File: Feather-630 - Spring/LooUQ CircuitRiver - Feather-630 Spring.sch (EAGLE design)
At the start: 22 parts, among them J1 FEATHERHOST-S, J2 FEATHERHOST-L, J3 HA-CTA_HEADER, J4 JST_PH-2_T/H, J5 JST_PH-2_T/H, P1 NO MOUNT, P2 NO MOUNT, P3 BREAKOUTPAD, U2 LM2674_BUCK

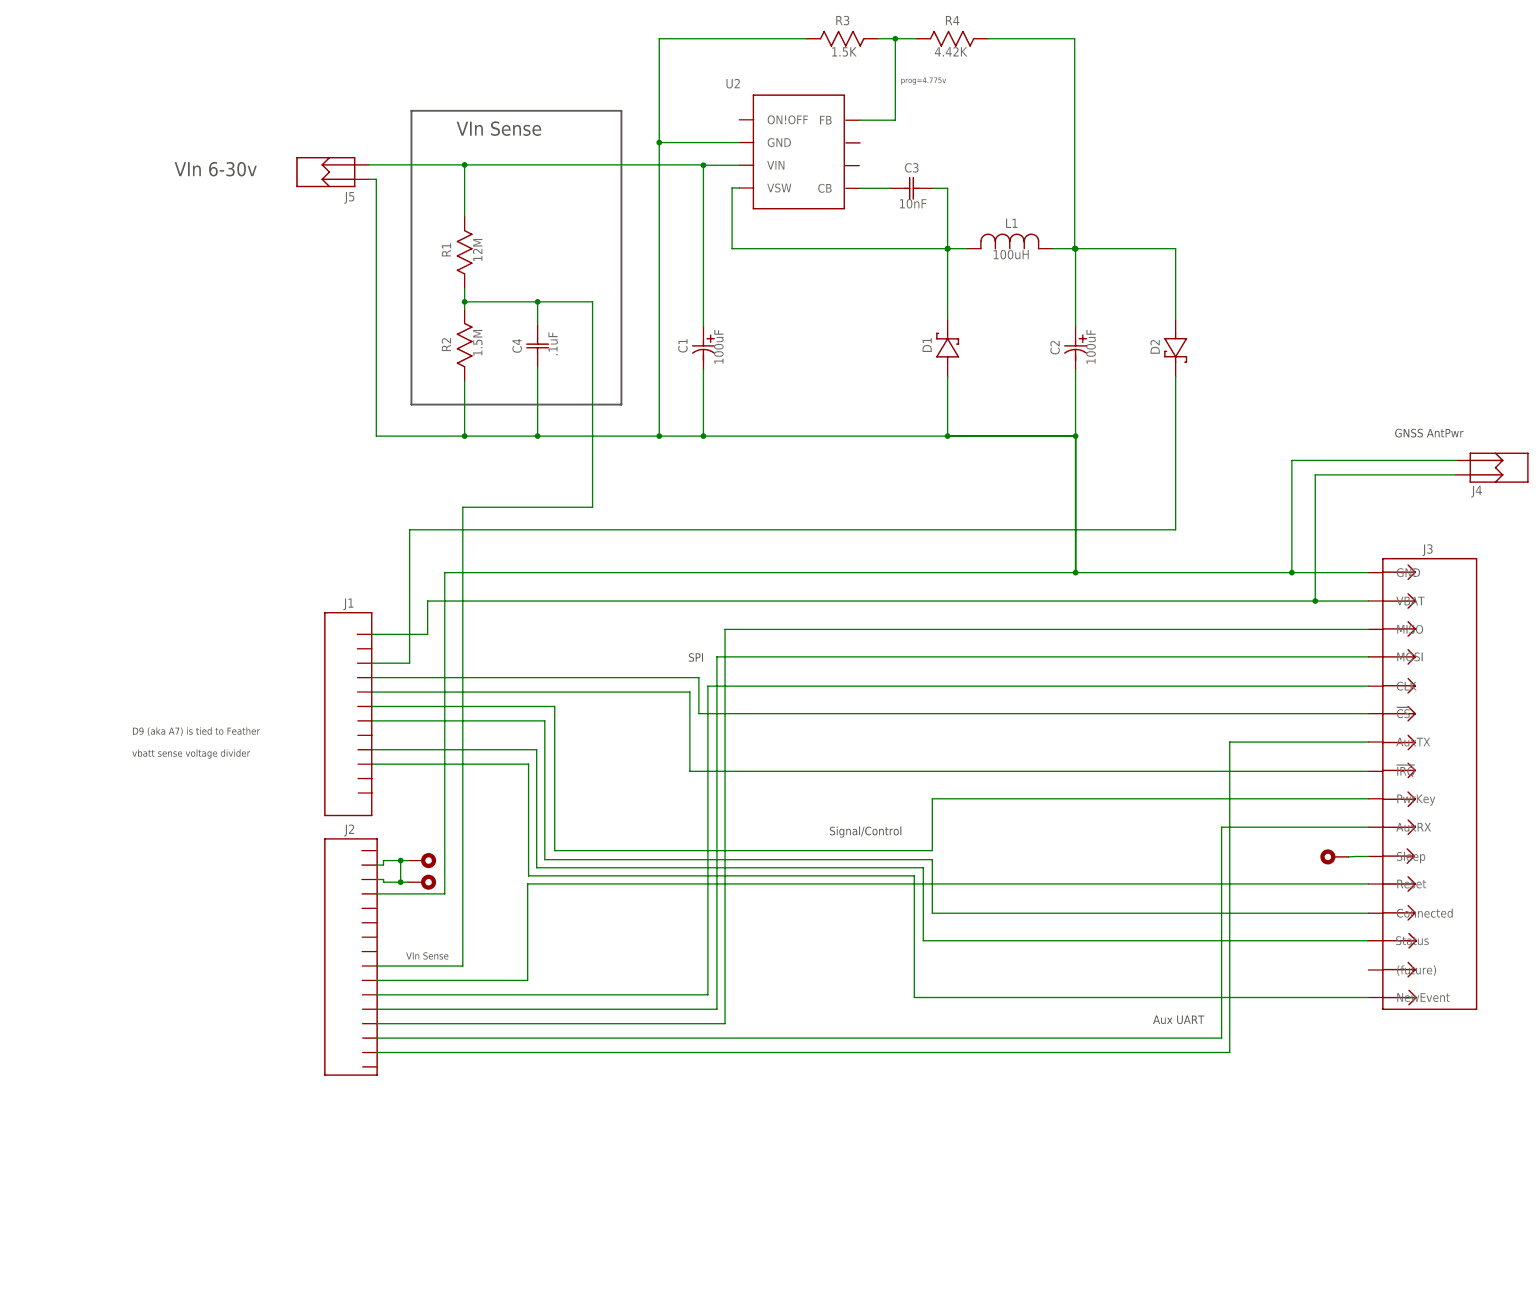
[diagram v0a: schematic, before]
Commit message: Updates for Feather-630
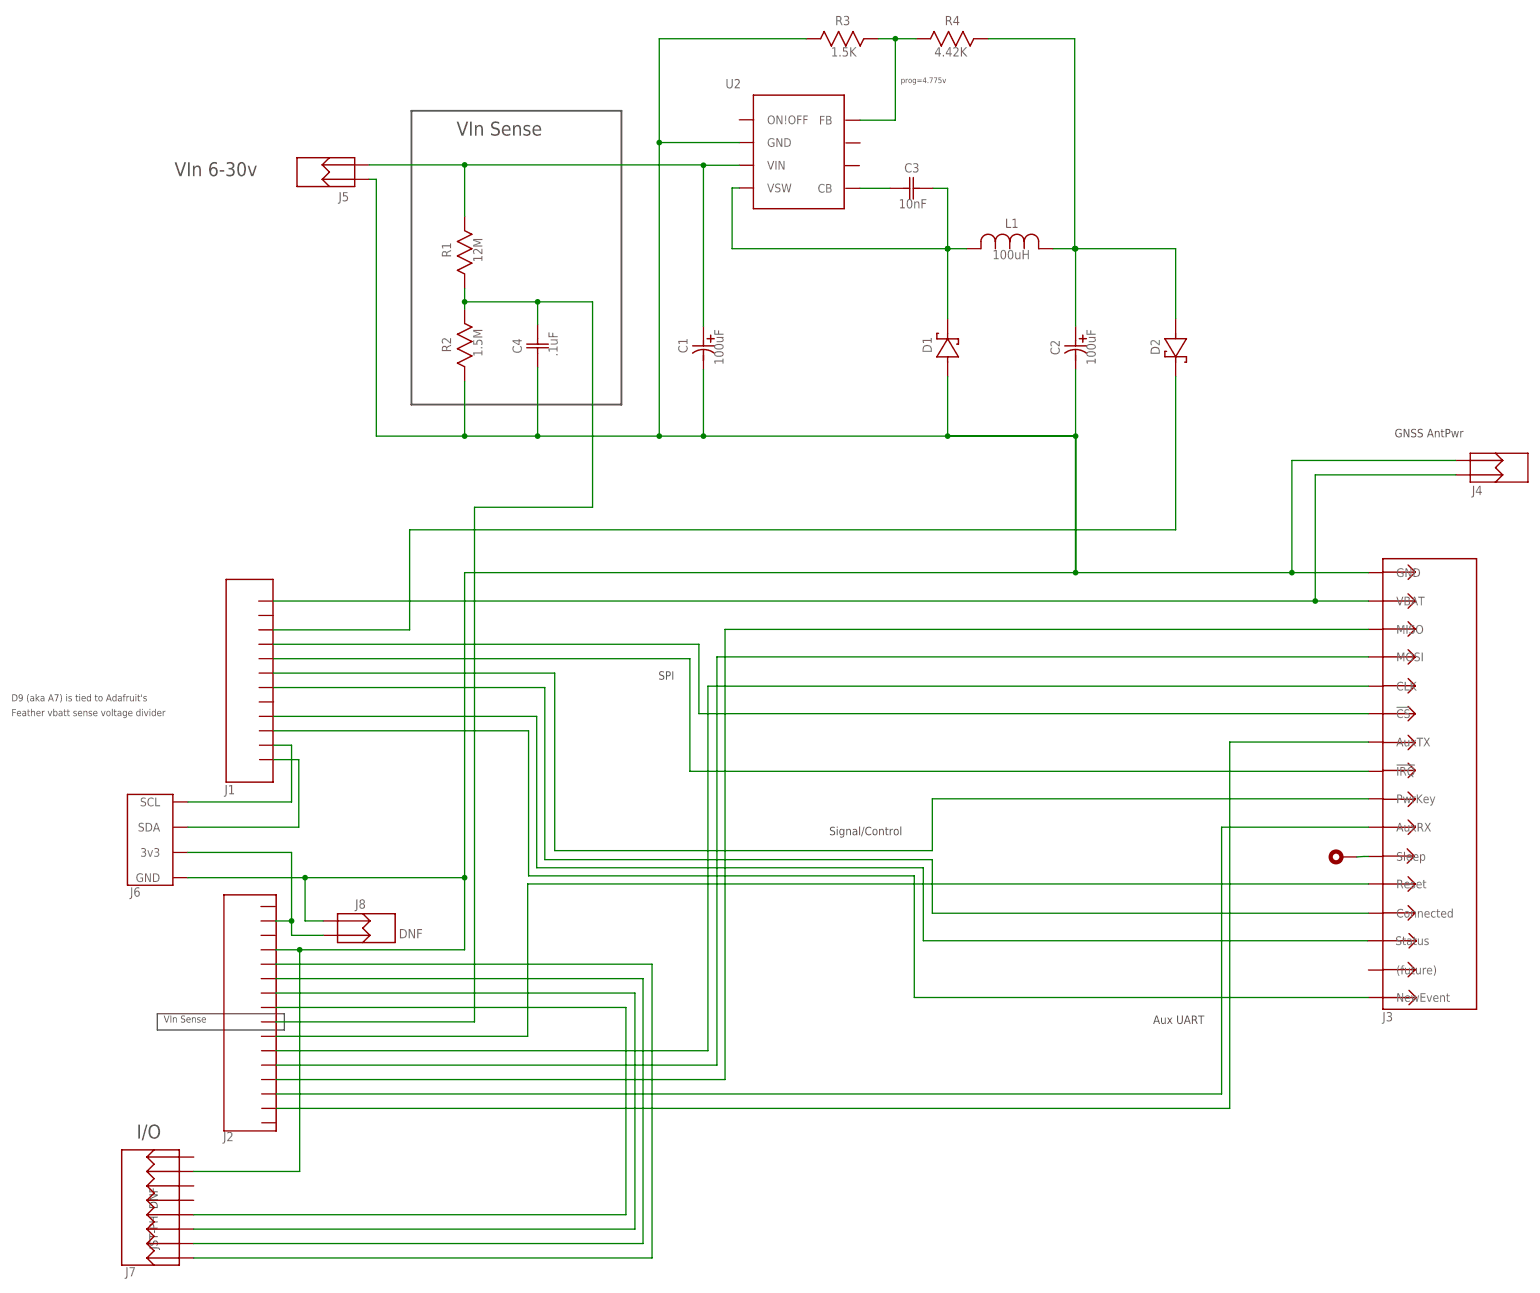
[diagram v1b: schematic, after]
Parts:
- removed P1, P2: NO MOUNT, common:BREAKOUTPAD
- added J6: QWIIC_VERTICAL, common:QWIIC_VERTICAL
- added J7: B8B-PH-K-S(LF)(SN), common:B8B-PH-K-S(LF)(SN)
- added J8: DNF, common:2PIN_T/H_HEADER
- J3: value HA-CTA_HEADER -> CR-SPRING_HEADER; device common:HA-CTA_HEADER -> common:CR-SPRING_HEADER
- P3: value BREAKOUTPAD -> SLEEP; device common:BREAKOUTPAD -> common:SLEEP
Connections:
- removed net Net_17: J2.+3V3, J2.AREF, P1.1, P2.1
- removed net Net_GND: C1.MINUS, C2.MINUS, C4.2, D1.A, J2.GND@2, J3.GND, J4.P2, J5.P2, R2.2, R3.1, U2.GND
- new net Net_11: J2.A0, J7.P8
- new net Net_23: J2.A3, J7.P5
- new net Net_24: J2.A2, J7.P6
- new net Net_25: J2.A1, J7.P7
- new net Net_27: J1.SDA, J6.SDA
- new net Net_28: J1.SCI, J6.SCL
- new net Net_29: J2.+3V3, J6.3v3, J8.P1
- new net Net_VIn: C1.PLUS, J5.P1, R1.2, U2.VIN
- net Net_13: now also C1.MINUS, C2.MINUS, C4.2, D1.A, J2.GND@2, J3.GND, J4.P2, J5.P2, J6.GND, J7.P2, J8.P2, R2.2, R3.1, U2.GND; no longer C1.PLUS, J5.P1, R1.2, U2.VIN
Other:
- note added: "D9 (aka A7) is tied to Adafruit's"
- note added: "Feather vbatt sense voltage divider"
- note added: "I/O"
- note added: "JST-PH DNF"
- note removed: "D9 (aka A7) is tied to Feather"
- note removed: "vbatt sense voltage divider"
- moved on the sheet: J1, J2
